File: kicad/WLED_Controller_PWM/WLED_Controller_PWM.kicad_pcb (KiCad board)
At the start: 2 copper layers, 72 x 50 mm, 63 parts, among them J1 USB_C_Receptacle_USB2.0, J5 Conn_01x05, J6 Conn_01x02, Q1 BC847, Q10 IRF540N, Q2 BC847, Q3 IRLL2705, Q4 IRLL2705, Q5 IRLL2705, Q6 IRLL2705, Q7 IRF540N, Q8 IRF540N, Q9 IRF540N, SW1 SW_RESET, SW2 SW_BOOT, SW3 SW_Push, U1 ESP32-WROOM-32, U2 CH340C, U3 NCP1117-3.3, U4 TSSP58P38, U5 L7805

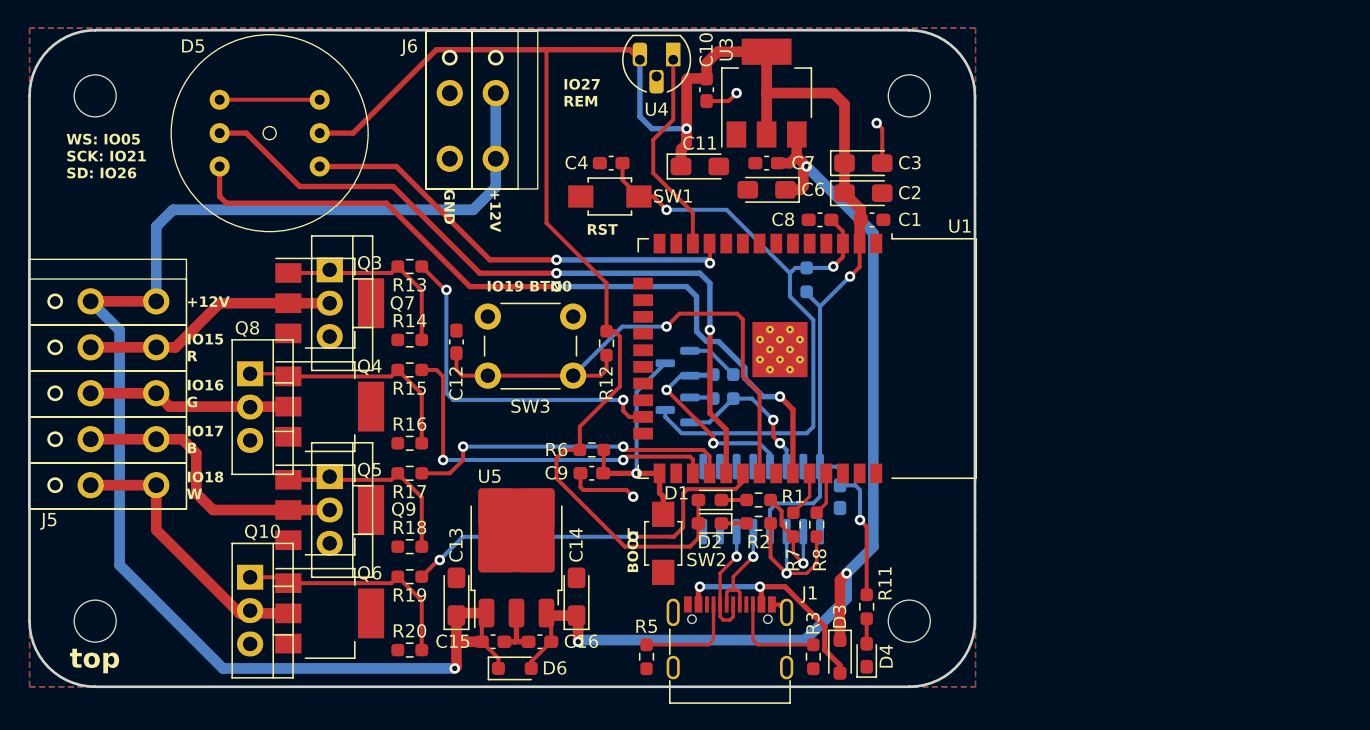
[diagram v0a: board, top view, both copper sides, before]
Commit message: Add new PCB-Layout
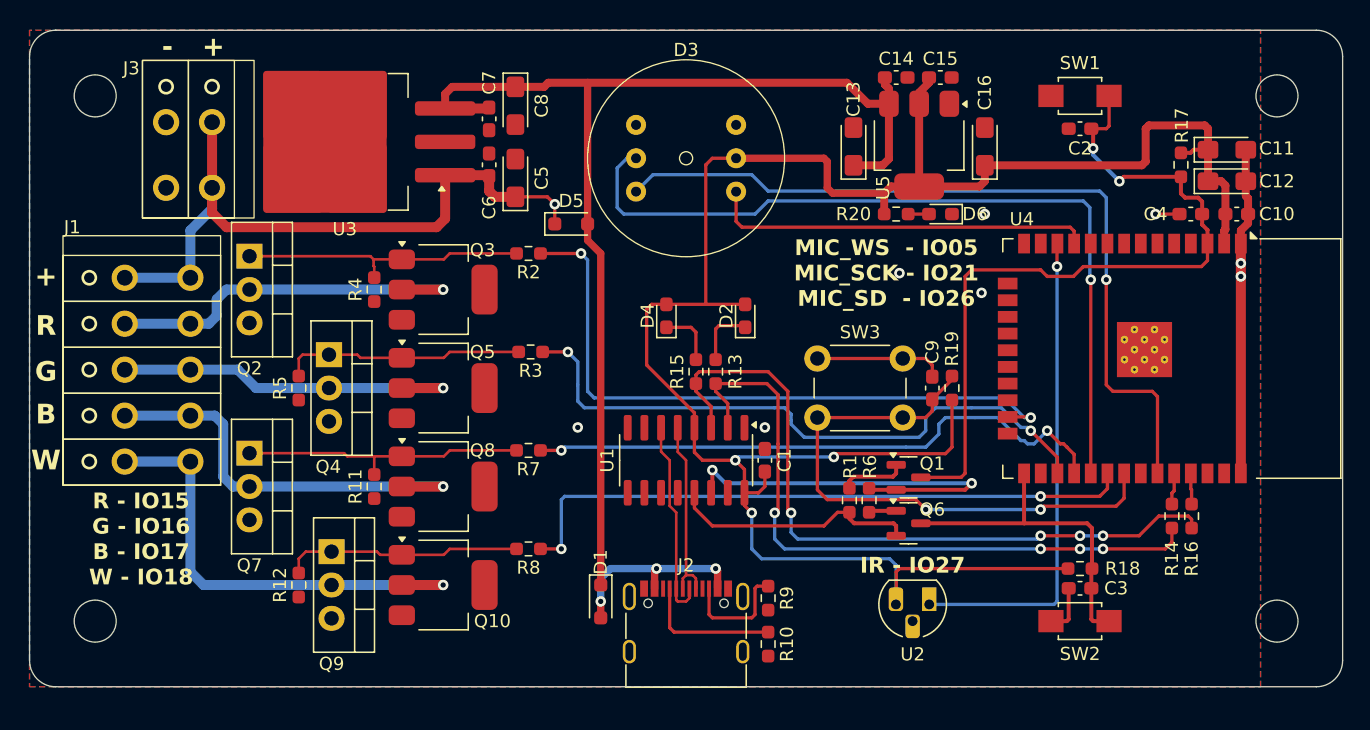
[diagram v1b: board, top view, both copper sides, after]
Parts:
- removed J5: Conn_01x05, GioN_Custom:WAGO_250-205_1x05_P3.50mm
- removed J6: Conn_01x02, GioN_Custom:WAGO_250-202_1x02_P3.50mm
- added J2: USB_C_Receptacle_USB2.0, GioN_Custom:USB_C, F.Cu at (50.0, -3.75)
- added J3: Conn_01x02, GioN_Custom:WAGO_250-202_1x02_P3.50mm, F.Cu at (8.60, -35.7)
- C12, C16, C8: value 100n -> 10u; footprint Capacitor_SMD:C_0603_1608Metric_Pad1.08x0.95mm_HandSolder -> Capacitor_Tantalum_SMD:CP_EIA-3216-18_Kemet-A_Pad1.58x1.35mm_HandSolder
- C14, C2, C3, C6: value 10u -> 100n; footprint Capacitor_Tantalum_SMD:CP_EIA-3216-18_Kemet-A_Pad1.58x1.35mm_HandSolder -> Capacitor_SMD:C_0603_1608Metric_Pad1.08x0.95mm_HandSolder
- C5: value 100n -> 10u; footprint Capacitor_SMD:C_0603_1608Metric_Pad1.08x0.95mm_HandSolder -> Capacitor_Tantalum_SMD:CP_EIA-3216-18_Kemet-A_Pad1.58x1.35mm_HandSolder; moved to F.Cu
- D1: value LED -> BAT60A; footprint LED_SMD:LED_0603_1608Metric_Pad1.05x0.95mm_HandSolder -> Diode_SMD:D_SOD-323_HandSoldering
- D3: value BAT60A -> INMP441; footprint Diode_SMD:D_SOD-323_HandSoldering -> GioN_Custom:INMP441_Module
- D5: value INMP441 -> BAT60A; footprint GioN_Custom:INMP441_Module -> Diode_SMD:D_SOD-323_HandSoldering
- D6: value BAT60A -> LED; footprint Diode_SMD:D_SOD-323_HandSoldering -> LED_SMD:LED_0603_1608Metric_Pad1.05x0.95mm_HandSolder
- J1: value USB_C_Receptacle_USB2.0 -> Conn_01x05; footprint GioN_Custom:USB_C -> GioN_Custom:WAGO_250-205_1x05_P3.50mm
- Q1, R4: moved to F.Cu
- Q10, Q8: value IRF540N -> IRLL2705; footprint Package_TO_SOT_THT:TO-220-3_Vertical -> Package_TO_SOT_SMD:SOT-223
- Q2: value BC847 -> IRF540N; footprint Package_TO_SOT_SMD:SOT-23 -> Package_TO_SOT_THT:TO-220-3_Vertical; moved to F.Cu
- Q4: value IRLL2705 -> IRF540N; footprint Package_TO_SOT_SMD:SOT-223 -> Package_TO_SOT_THT:TO-220-3_Vertical
- Q6: value IRLL2705 -> BC847; footprint Package_TO_SOT_SMD:SOT-223 -> Package_TO_SOT_SMD:SOT-23
- R1: value 1k -> 10k
- R10, R9: value 10k -> 5k1; moved to F.Cu
- R11: value 220R -> 10k
- R13, R15: value 100R -> 1k
- R14, R16: value 10k -> 100R
- R17, R19: value 100R -> 10k
- R18: value 10k -> 5k
- R2: value 1k -> 100R
- R20: value 10k -> 220R
- R3: value 5k1 -> 100R
- R5: value 5k1 -> 10k
- R6: value 5k -> 10k
- U1: value ESP32-WROOM-32 -> CH340C; footprint RF_Module:ESP32-WROOM-32 -> Package_SO:SOIC-16_3.9x9.9mm_P1.27mm
- U2: value CH340C -> TSSP58P38; footprint Package_SO:SOIC-16_3.9x9.9mm_P1.27mm -> Package_TO_SOT_THT:TO-92L_HandSolder; moved to F.Cu
- U3: value NCP1117-3.3 -> L7805; footprint Package_TO_SOT_SMD:SOT-223-3_TabPin2 -> Package_TO_SOT_SMD:TO-263-3_TabPin2
- U4: value TSSP58P38 -> ESP32-WROOM-32; footprint Package_TO_SOT_THT:TO-92L_HandSolder -> RF_Module:ESP32-WROOM-32
- U5: value L7805 -> NCP1117-3.3; footprint Package_TO_SOT_SMD:TO-252-3_TabPin2 -> Package_TO_SOT_SMD:SOT-223-3_TabPin2
- moved R17 63.3 mm to (87.7, -39.8), turned to -90 degrees
- moved C12 59.9 mm to (91.2, -38.5), turned to 0 degrees
- moved R16 59.8 mm to (88.5, -13.0), turned to 90 degrees
- moved R14 59.6 mm to (87.0, -13.0), turned to 90 degrees
- moved C15 54.8 mm to (69.4, -46.4)
- moved R18 51.1 mm to (80.0, -9.00)
- moved C16 50.7 mm to (72.8, -41.1), turned to 90 degrees
- moved R20 49.7 mm to (66.0, -36.0)
- moved D6 47.4 mm to (69.4, -36.0), turned to 180 degrees
- moved C14 46.4 mm to (66.0, -46.4), turned to 0 degrees
- moved C13 45.7 mm to (62.8, -41.1)
- moved Q6 44.6 mm to (66.9, -12.4)
- moved C4 44.3 mm to (88.4, -36.0)
- moved R19 43.7 mm to (70.2, -22.8), turned to 90 degrees
- moved U5 43.3 mm to (67.8, -41.2), turned to -90 degrees
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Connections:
- C12 pad 1: GND -> +3.3V
- C12 pad 2: Button0 -> GND
- C13 pad 1: +12V -> +5V
- C15 pad 1: +12V -> +3.3V
- C16 pad 1: +5V -> +3.3V
- C2 pad 1: +3.3V -> GND
- C2 pad 2: GND -> ESP_EN
- C3 pad 1: +3.3V -> GND
- C3 pad 2: GND -> ESP_IO0
- C5 pad 1: +3.3V -> +12V
- C6 pad 1: +5V -> +12V
- C8 pad 1: GND -> +5V
- C8 pad 2: ESP_EN -> GND
- C9 pad 2: ESP_IO0 -> Button0
- D1 pad 1: Net-(D1-K) -> +5V
- D1 pad 2: +3.3V -> Net-(D1-A)
- D3 pad 1: +5V -> GND
- D3 pad 2: Net-(D3-A) -> MIC_WS
- D4 pad 1: GND -> Net-(D4-K)
- D4 pad 2: Net-(D4-A) -> +3.3V
- D5 pad 1: GND -> +12V
- D5 pad 2: MIC_WS -> +5V
- D6 pad 1: +12V -> GND
- D6 pad 2: +5V -> Net-(D6-A)
- Q10 pad 2: Net-(J5-Pin_5) -> Net-(J1-Pin_5)
- Q2 pad 1: Net-(Q2-B) -> Net-(Q2-G)
- Q2 pad 2: ~{DTR} -> Net-(J1-Pin_2)
- Q2 pad 3: ESP_IO0 -> GND
- Q3 pad 1: Net-(Q3-G) -> Net-(Q2-G)
- Q3 pad 2: Net-(J5-Pin_2) -> Net-(J1-Pin_2)
- Q4 pad 2: Net-(J5-Pin_3) -> Net-(J1-Pin_3)
- Q5 pad 1: Net-(Q5-G) -> Net-(Q4-G)
- Q5 pad 2: Net-(J5-Pin_4) -> Net-(J1-Pin_3)
- Q6 pad 1: Net-(Q10-G) -> Net-(Q6-B)
- Q6 pad 2: Net-(J5-Pin_5) -> ~{DTR}
- Q6 pad 3: GND -> ESP_IO0
- Q7 pad 1: Net-(Q3-G) -> Net-(Q7-G)
- Q7 pad 2: Net-(J5-Pin_2) -> Net-(J1-Pin_4)
- Q8 pad 1: Net-(Q4-G) -> Net-(Q7-G)
- Q8 pad 2: Net-(J5-Pin_3) -> Net-(J1-Pin_4)
- Q9 pad 1: Net-(Q5-G) -> Net-(Q10-G)
- Q9 pad 2: Net-(J5-Pin_4) -> Net-(J1-Pin_5)
- R1 pad 1: TX -> ~{DTR}
- R1 pad 2: Net-(D1-K) -> Net-(Q1-B)
- R10 pad 1: ~{RTS} -> Net-(J2-CC1)
- R10 pad 2: Net-(Q2-B) -> GND
- R11 pad 1: +3.3V -> GND
- R11 pad 2: Net-(D4-A) -> Net-(Q7-G)
- R12 pad 1: +3.3V -> GND
- R12 pad 2: Button0 -> Net-(Q10-G)
- R13 pad 1: LED_R -> TX
- R13 pad 2: Net-(Q3-G) -> Net-(D2-K)
- R14 pad 1: GND -> TX
- R14 pad 2: Net-(Q3-G) -> ESP_RX
- R15 pad 1: LED_G -> RX
- R15 pad 2: Net-(Q4-G) -> Net-(D4-K)
- R16 pad 1: GND -> RX
- R16 pad 2: Net-(Q4-G) -> ESP_TX
- R17 pad 1: LED_B -> +3.3V
- R17 pad 2: Net-(Q5-G) -> ESP_EN
- R18 pad 1: GND -> +3.3V
- R18 pad 2: Net-(Q5-G) -> ESP_IO0
- R19 pad 1: LED_W -> +3.3V
- R19 pad 2: Net-(Q10-G) -> Button0
- R2 pad 1: RX -> LED_R
- R2 pad 2: Net-(D2-K) -> Net-(Q2-G)
- R20 pad 1: GND -> +3.3V
- R20 pad 2: Net-(Q10-G) -> Net-(D6-A)
- R3 pad 1: Net-(J1-CC2) -> LED_G
- R3 pad 2: GND -> Net-(Q4-G)
- R4 pad 1: +3.3V -> GND
- R4 pad 2: ESP_EN -> Net-(Q2-G)
- R5 pad 1: Net-(J1-CC1) -> GND
- R5 pad 2: GND -> Net-(Q4-G)
- R6 pad 1: +3.3V -> ~{RTS}
- R6 pad 2: ESP_IO0 -> Net-(Q6-B)
- R7 pad 1: TX -> LED_B
- R7 pad 2: ESP_RX -> Net-(Q7-G)
- R8 pad 1: RX -> LED_W
- R8 pad 2: ESP_TX -> Net-(Q10-G)
- R9 pad 1: ~{DTR} -> Net-(J2-CC2)
- R9 pad 2: Net-(Q1-B) -> GND
- U1 pad 10: IO25 -> unconnected-(U1-~{DSR}-Pad10)
- U1 pad 11: MIC_SD -> unconnected-(U1-~{RI}-Pad11)
- U1 pad 12: SENSE0 -> unconnected-(U1-~{DCD}-Pad12)
- U1 pad 13: IO14 -> ~{DTR}
- U1 pad 14: IO12 -> ~{RTS}
- U1 pad 15: GND -> unconnected-(U1-R232-Pad15)
- U1 pad 16: IO13 -> +3.3V
- U1 pad 2: +3.3V -> TX
- U1 pad 3: ESP_EN -> RX
- U1 pad 4: unconnected-(U1-SENSOR_VP-Pad4) -> +3.3V
- U1 pad 5: unconnected-(U1-SENSOR_VN-Pad5) -> D+
- U1 pad 6: IO34 -> D-
- U1 pad 7: IO35 -> unconnected-(U1-NC-Pad7)
- U1 pad 8: IO32 -> unconnected-(U1-NC-Pad8)
- U1 pad 9: IO33 -> unconnected-(U1-~{CTS}-Pad9)
- U2 pad 1: GND -> SENSE0
- U2 pad 2: TX -> GND
- U2 pad 3: RX -> +3.3V
- U3 pad 1: GND -> +12V
- U3 pad 2: +3.3V -> GND
- U4 pad 1: SENSE0 -> GND
- U4 pad 2: GND -> +3.3V
- U4 pad 3: +3.3V -> ESP_EN
- U5 pad 1: +12V -> GND
- U5 pad 2: GND -> +3.3V
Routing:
- net +12V: track 108.1 -> 52.7 mm
- net TX: track 8.27 -> 51.8 mm, vias 1 -> 4
- net RX: track 12.1 -> 55.3 mm, vias 1 -> 4
- net Net-(J1-Pin_5): track 0.00 -> 36.2 mm, vias 0 -> 1
- net Net-(J1-Pin_4): track 0.00 -> 32.0 mm, vias 0 -> 1
- net Net-(J1-Pin_2): track 0.00 -> 29.2 mm, vias 0 -> 1
- net Net-(J1-Pin_3): track 0.00 -> 28.0 mm, vias 0 -> 1
- net LED_R: track 26.7 -> 50.2 mm
- net Net-(J5-Pin_4): track 22.2 -> 0.00 mm
- net Net-(Q2-G): track 0.00 -> 22.0 mm
- net Net-(Q7-G): track 0.00 -> 22.0 mm
- net SENSE0: track 15.9 -> 37.1 mm, vias 0 -> 1
- net Net-(J5-Pin_5): track 21.1 -> 0.00 mm
- net LED_B: track 25.0 -> 45.6 mm
- net LED_G: track 28.5 -> 48.4 mm
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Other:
- board size 72 x 50 mm -> 100 x 50 mm
- board text added: "+"
- board text added: "-"
- board text added: "B"
- board text added: "G"
- board text added: "IR - IO27"
- board text added: "MIC_WS - IO05 MIC_SCK - IO21 MIC_SD - IO26"
- board text added: "R"
- board text added: "R - IO15 G - IO16 B - IO17 W - IO18"
- board text added: "W"
- board text added: "WLED-Controller (PWM) Ver.1 Rev.0 02/25 Gioulekas Nikos"
- board text removed: "+12V"
- board text removed: "BOOT"
- board text removed: "GND"
- board text removed: "IO15 R"
- board text removed: "IO16 G"
- board text removed: "IO17 B"
- board text removed: "IO18 W"
- board text removed: "IO19 BTN0"
- board text removed: "IO27 REM"
- board text removed: "RST"
- board text removed: "WLED Controller PWM V1 R1 05/2024 Gioulekas Nikos"
- board text removed: "WS: IO05 SCK: IO21 SD: IO26"
- board text removed: "bot"
- board text removed: "top"
